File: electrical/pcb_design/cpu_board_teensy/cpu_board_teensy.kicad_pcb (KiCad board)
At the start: 2 copper layers, 82.5 x 82.5 mm, 9 parts, among them J1 Molex_504050-1291, M1 M3, M2 M3, M3 M3, M4 M3, U1 Teensy4.0_TopPinsOnly, U2 RFM69HCW, U3 BNO085_Adafruit_Breakout_I2C, U4 BMP390_Adafruit_Breakout

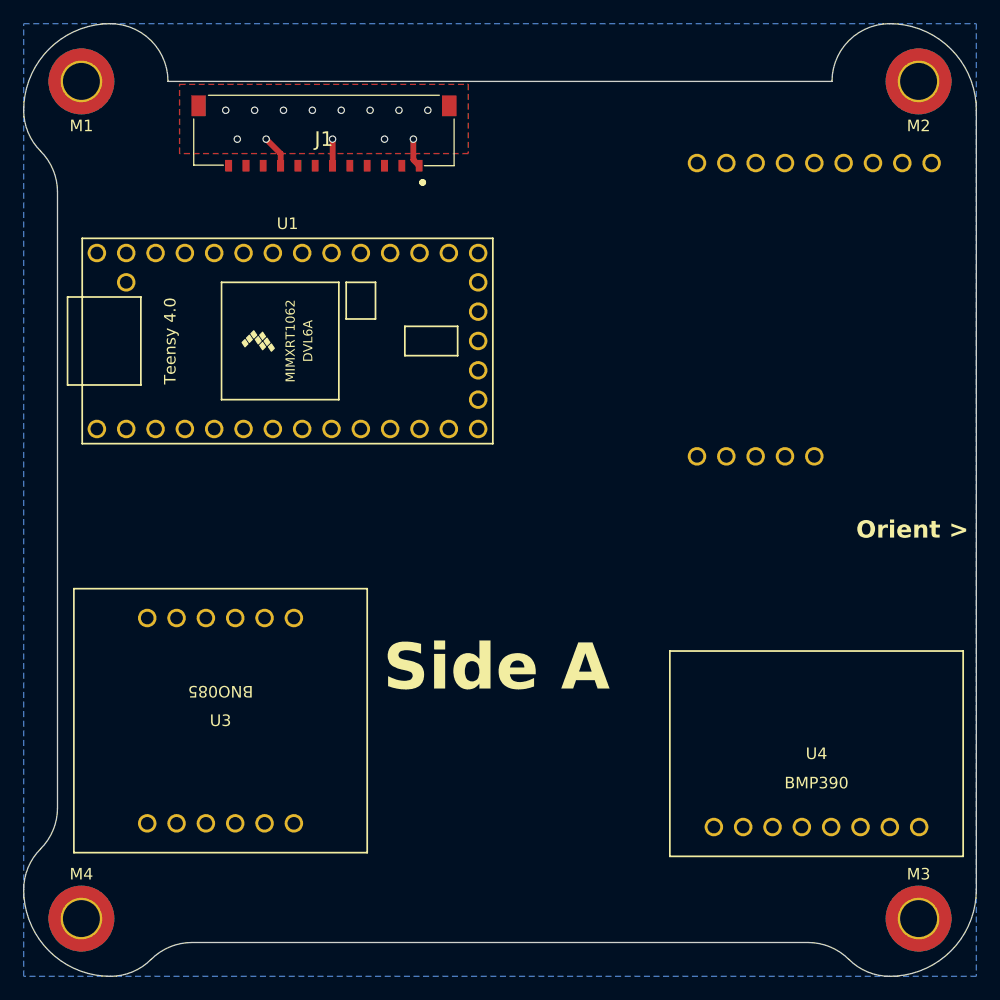
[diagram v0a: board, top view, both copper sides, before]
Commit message: Finished iteration on Teensy CPU board
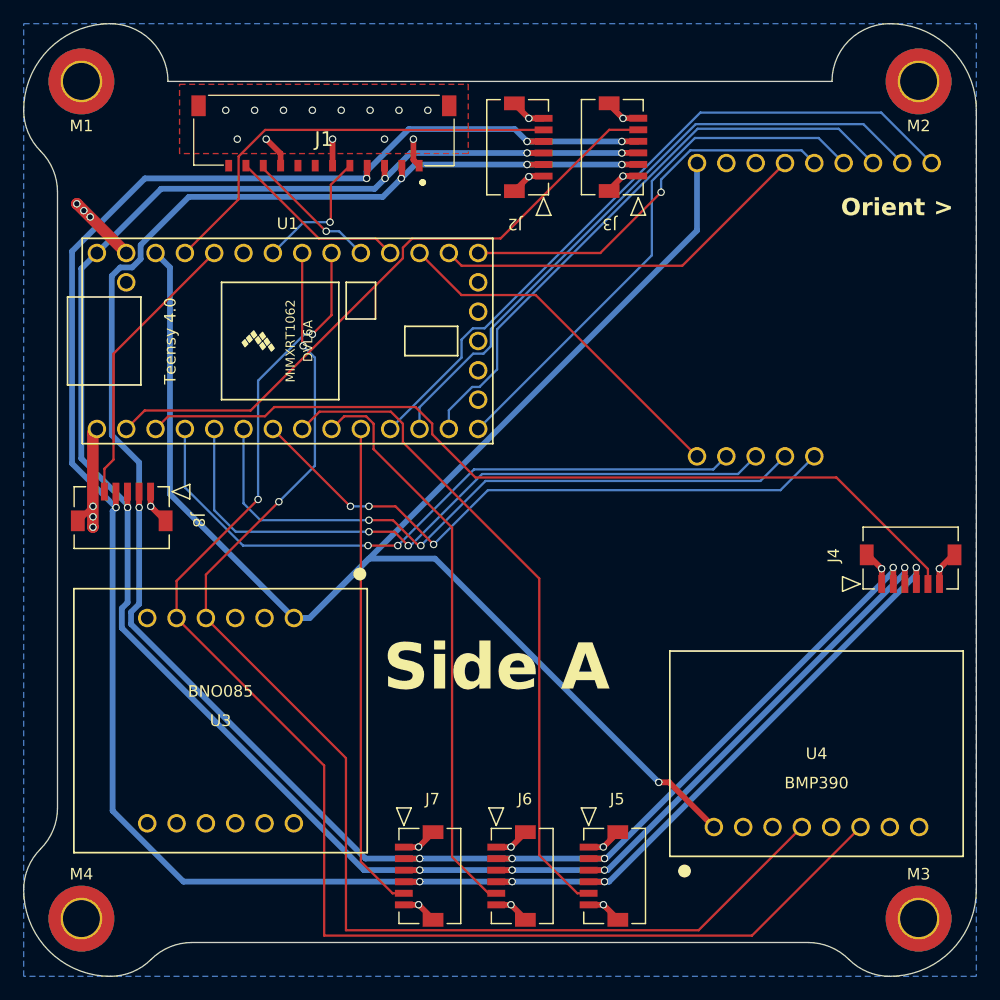
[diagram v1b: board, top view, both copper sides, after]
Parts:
- added J2: HEATER_PWM, footprints:Molex_5013310607, F.Cu at (142.5, 78.5)
- added J3: MAGNETORQUER_PWM_0, footprints:Molex_5013310607, F.Cu at (150.8, 78.5)
- added J4: MAGNETORQUER_PWM_1, footprints:Molex_5013310607, F.Cu at (176.5, 113.5)
- added J5: MAGNETORQUER_PWM_2, footprints:Molex_5013310607, F.Cu at (151.4, 141.0)
- added J6: MAGNETORQUER_PWM_3, footprints:Molex_5013310607, F.Cu at (143.4, 141.0)
- added J7: MAGNETORQUER_PWM_4, footprints:Molex_5013310607, F.Cu at (135.4, 141.0)
- added J8: MAGNETORQUER_PWM_5, footprints:Molex_5013310607, F.Cu at (108.8, 110.5)
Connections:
- J1 pad 2: unconnected-(J1-Pad2) -> VCC
- J1 pad 4: unconnected-(J1-Pad4) -> +3.3VA
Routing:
- net +3.3VA: track 0.00 -> 197.6 mm, vias 0 -> 8
- net +5V: track 0.00 -> 182.5 mm, vias 0 -> 8
- net VCC: track 0.00 -> 176.3 mm, vias 0 -> 8
- net +3V3: track 0.00 -> 139.4 mm, vias 0 -> 1
- net LOCAL_SDA: track 0.00 -> 120.7 mm, vias 0 -> 2
- net LOCAL_SCL: track 0.00 -> 111.2 mm, vias 0 -> 2
- net /MAG_PWM_1: track 0.00 -> 75.3 mm
- net /RADIO_RESET: track 0.00 -> 61.0 mm
- net GND: track 7.62 -> 66.6 mm, vias 13 -> 32
- net /GPIO_3: track 0.00 -> 58.4 mm, vias 0 -> 2
- net /GPIO_4: track 0.00 -> 58.0 mm, vias 0 -> 2
- net /MAG_PWM_2: track 0.00 -> 57.7 mm
- net /GPIO_2: track 0.00 -> 57.2 mm, vias 0 -> 2
- net /CS: track 0.00 -> 56.1 mm
- net /MAG_PWM_0: track 0.00 -> 55.6 mm
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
